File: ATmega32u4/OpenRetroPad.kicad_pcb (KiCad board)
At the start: 2 copper layers, 46 x 74 mm, 56 parts, among them J1 USB_C_Receptacle_USB2.0, J2 NRF24, J3 DB25_Female_MountingHoles, J4 USB_C_Receptacle_USB2.0, SW1 SW_Push, SW2 SW_Push, U1 ATmega32U4, U2 AMS1117-3.3, U3 CH330N, Y1 16MHz

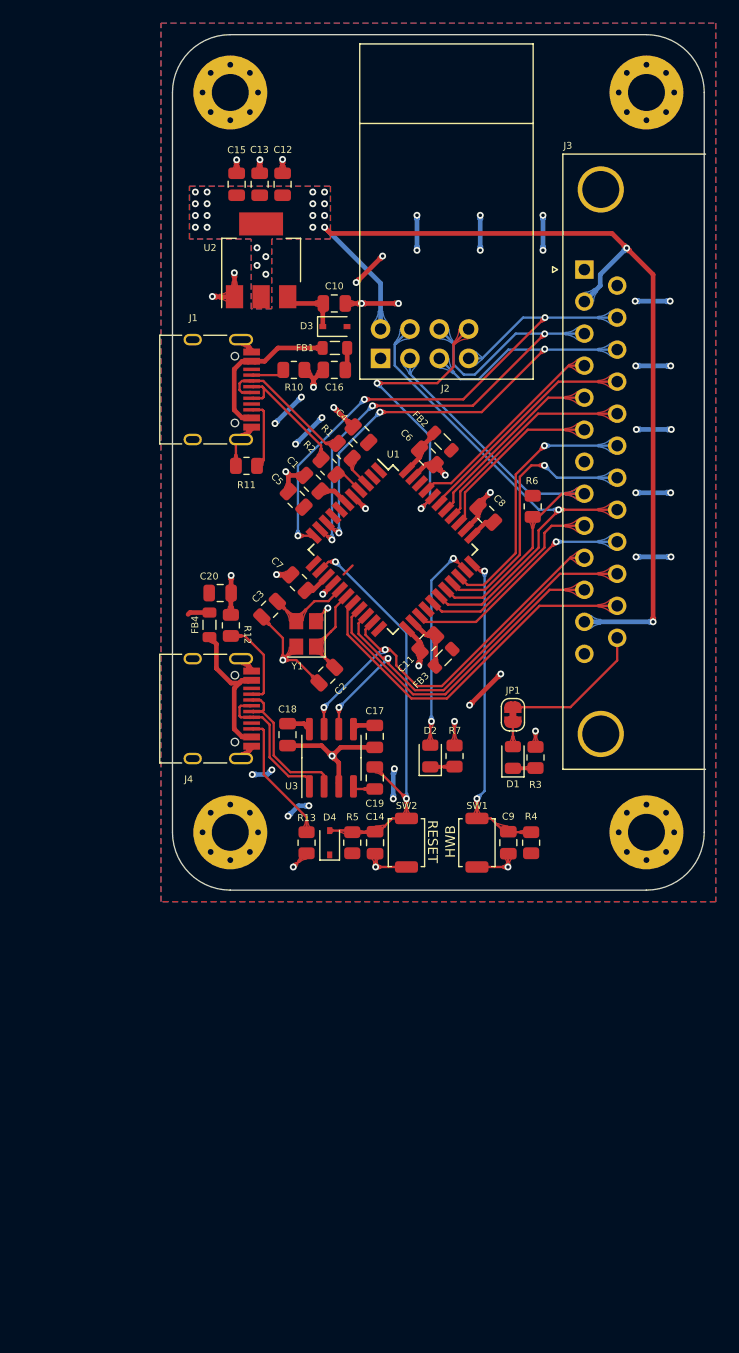
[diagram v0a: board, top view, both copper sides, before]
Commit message: Update V2
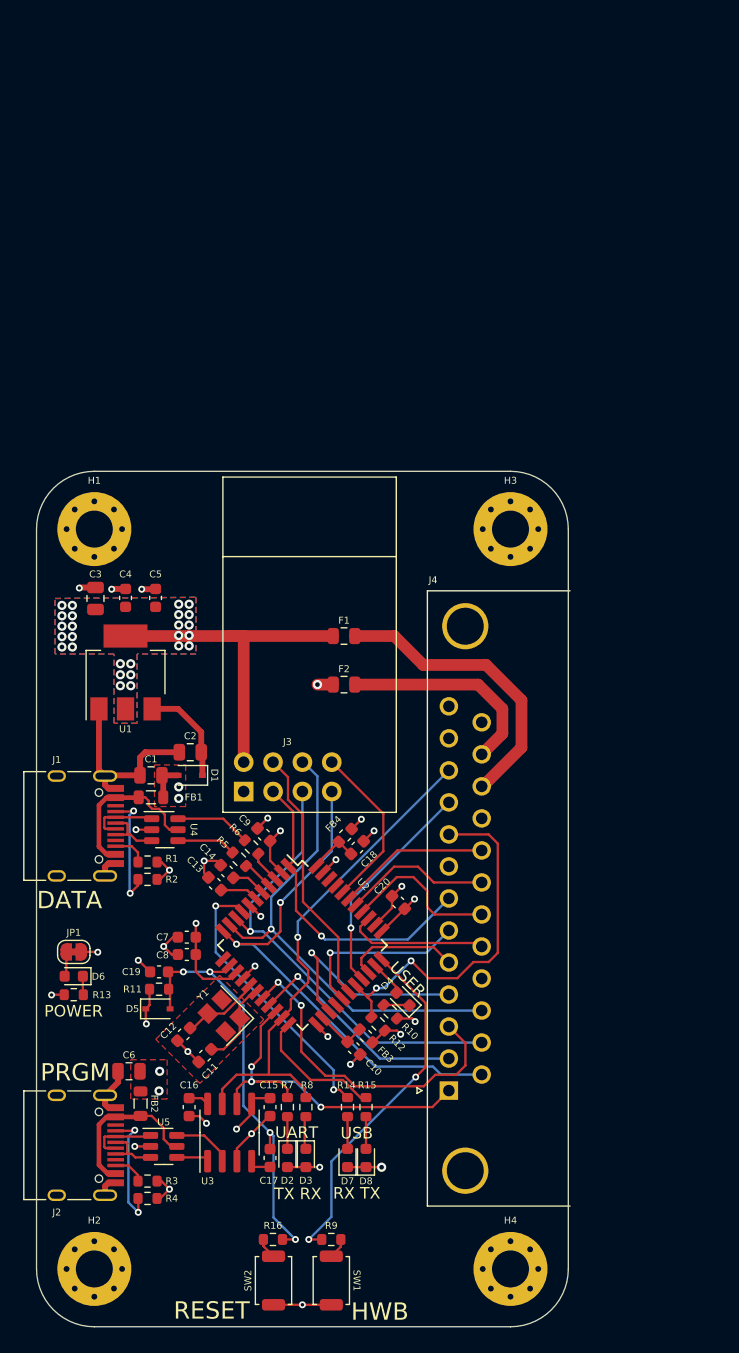
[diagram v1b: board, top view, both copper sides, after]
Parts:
- added D5: 1N5817, Diode_SMD:D_SOD-323, F.Cu at (105.5, 141.5)
- added D6: Power, LED_SMD:LED_0603_1608Metric, F.Cu at (98.2, 138.7)
- added D7: RX, LED_SMD:LED_0603_1608Metric, F.Cu at (121.9, 154.4)
- added D8: TX, LED_SMD:LED_0603_1608Metric, F.Cu at (123.5, 154.4)
- added F1: 500mA, Fuse:Fuse_0805_2012Metric, F.Cu at (121.6, 109.2)
- added F2: 500mA, Fuse:Fuse_0805_2012Metric, F.Cu at (121.6, 113.5)
- added R14: 1k, Resistor_SMD:R_0603_1608Metric, F.Cu at (121.9, 150.0)
- added R15: 1k, Resistor_SMD:R_0603_1608Metric, F.Cu at (123.5, 150.0)
- added R16: 330, Resistor_SMD:R_0603_1608Metric, F.Cu at (115.5, 161.4)
- added R8: 1k, Resistor_SMD:R_0603_1608Metric, F.Cu at (118.3, 150.0)
- added R9: 330, Resistor_SMD:R_0603_1608Metric, F.Cu at (120.5, 161.4)
- added U4: USBLC6-2SC6, Package_TO_SOT_SMD:SOT-23-6, F.Cu at (106.1, 126.0)
- added U5: USBLC6-2SC6, Package_TO_SOT_SMD:SOT-23-6, F.Cu at (106.0, 153.4)
- C1: value 1u -> 10u
- C10, C16, C20: value 10u -> 100n; footprint Capacitor_SMD:C_0805_2012Metric -> Capacitor_SMD:C_0603_1608Metric
- C11: value 100n -> 20pF; footprint Capacitor_SMD:C_0805_2012Metric -> Capacitor_SMD:C_0603_1608Metric
- C12: value 10u -> 20pF; footprint Capacitor_SMD:C_0805_2012Metric -> Capacitor_SMD:C_0603_1608Metric
- C13, C15, C17, C18, C19, C4, C8, C9: footprint Capacitor_SMD:C_0805_2012Metric -> Capacitor_SMD:C_0603_1608Metric
- C14, C7: value 100n -> 1u; footprint Capacitor_SMD:C_0805_2012Metric -> Capacitor_SMD:C_0603_1608Metric
- C2, C3: value 20pF -> 10u
- C5: value 1u -> 100n; footprint Capacitor_SMD:C_0805_2012Metric -> Capacitor_SMD:C_0603_1608Metric
- C6: value 100n -> 10u
- D1: value Power LED -> 1N5817; footprint LED_SMD:LED_0805_2012Metric -> Diode_SMD:D_SOD-323
- D2: value LED1 -> TX; footprint LED_SMD:LED_0805_2012Metric -> LED_SMD:LED_0603_1608Metric
- D3: value 1N5817 -> RX; footprint Diode_SMD:D_SOD-323 -> LED_SMD:LED_0603_1608Metric
- D4: value 1N5817 -> User; footprint Diode_SMD:D_SOD-323 -> LED_SMD:LED_0603_1608Metric
- FB3, FB4: footprint Inductor_SMD:L_0805_2012Metric -> Inductor_SMD:L_0603_1608Metric
- H1, H2, H3, H4: value 3.2mm_M3 -> 3.2mm M3
- J2: value NRF24 -> USB_C_Receptacle_USB2.0; footprint OpenRetroPad:NRF24L01 -> Connector_USB:USB_C_Receptacle_HRO_TYPE-C-31-M-12
- J3: value DB25_Female_MountingHoles -> NRF24; footprint Connector_Dsub:DSUB-25_Female_Horizontal_P2.77x2.84mm_EdgePinOffset7.70mm_Housed_MountingHolesOffset9.12mm -> OpenRetroPad:NRF24L01
- J4: value USB_C_Receptacle_USB2.0 -> DB25_Male_MountingHoles; footprint Connector_USB:USB_C_Receptacle_HRO_TYPE-C-31-M-12 -> Connector_Dsub:DSUB-25_Male_Horizontal_P2.77x2.84mm_EdgePinOffset7.70mm_Housed_MountingHolesOffset9.12mm
- R1, R2: value 22r -> 5.1k; footprint Resistor_SMD:R_0805_2012Metric -> Resistor_SMD:R_0603_1608Metric
- R10, R12, R13: value 5.1k -> 1k; footprint Resistor_SMD:R_0805_2012Metric -> Resistor_SMD:R_0603_1608Metric
- R11: value 5.1k -> 10k; footprint Resistor_SMD:R_0805_2012Metric -> Resistor_SMD:R_0603_1608Metric
- R3: value 1k -> 5.1k; footprint Resistor_SMD:R_0805_2012Metric -> Resistor_SMD:R_0603_1608Metric
- R4: value 10k -> 5.1k; footprint Resistor_SMD:R_0805_2012Metric -> Resistor_SMD:R_0603_1608Metric
- R5: value 10k -> 22r; footprint Resistor_SMD:R_0805_2012Metric -> Resistor_SMD:R_0603_1608Metric
- R6: value 1k -> 22r; footprint Resistor_SMD:R_0805_2012Metric -> Resistor_SMD:R_0603_1608Metric
- R7: footprint Resistor_SMD:R_0805_2012Metric -> Resistor_SMD:R_0603_1608Metric
- SW1: value SW_Push -> HWB
- SW2: value SW_Push -> RESET
- U1: value ATmega32U4 -> AMS1117-3.3; footprint Package_QFP:TQFP-44_10x10mm_P0.8mm -> Package_TO_SOT_SMD:SOT-223-3_TabPin2
- U2: value AMS1117-3.3 -> ATmega32U4-M; footprint Package_TO_SOT_SMD:SOT-223-3_TabPin2 -> Package_QFP:TQFP-44_10x10mm_P0.8mm
- moved H2 112.4 mm to (100.0, 164.0)
- moved C15 79.9 mm to (115.2, 150.0), turned to 90 degrees
- moved C12 74.0 mm to (107.7, 143.7), turned to -135 degrees
- moved J2 73.2 mm to (97.8, 153.3), turned to -90 degrees
- moved D3 72.0 mm to (118.3, 154.4), turned to -90 degrees
- moved C16 65.0 mm to (108.2, 150.0), turned to 90 degrees
- moved C10 64.4 mm to (122.5, 144.9), turned to 135 degrees
- moved FB2 63.0 mm to (104.0, 149.7), turned to 90 degrees
- moved C13 60.6 mm to (110.4, 130.7), turned to -45 degrees
- moved U2 59.4 mm to (118.0, 136.0), turned to -45 degrees
- moved C6 59.1 mm to (103.0, 146.9), turned to 0 degrees
- moved R10 56.1 mm to (125.6, 141.8), turned to 135 degrees
- moved J3 53.9 mm to (112.9, 122.7)
- moved R3 49.7 mm to (104.6, 156.4), turned to 0 degrees
- moved LOGO1 46.3 mm to (109.1, 164.1)
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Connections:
- C1 pad 2: Net-(C1-Pad2) -> +5V
- C10 pad 2: Net-(C10-Pad2) -> /Microcontroller/AVCC_P24
- C11 pad 1: GND -> /Microcontroller/XTAL1
- C11 pad 2: Net-(C11-Pad2) -> GND
- C12 pad 1: GND -> /Microcontroller/XTAL2
- C12 pad 2: +3V3 -> GND
- C13 pad 2: +3V3 -> /Microcontroller/UCAP
- C14 pad 1: RESET -> GND
- C14 pad 2: GND -> /Microcontroller/UGND
- C15 pad 2: +3V3 -> +5V
- C16 pad 2: +5V -> /UART/V3
- C17 pad 1: GND -> /UART/RTS
- C17 pad 2: +5V -> /DB25/RST
- C18 pad 2: Net-(C18-Pad2) -> /Microcontroller/AVCC_P44
- C19 pad 1: Net-(C19-Pad1) -> /DB25/RST
- C19 pad 2: RESET -> GND
- C2 pad 1: XTAL1 -> GND
- C2 pad 2: GND -> /Power/VREGIN
- C3 pad 1: XTAL2 -> GND
- C3 pad 2: GND -> +3V3
- C4 pad 2: +5V -> +3V3
- C5 pad 2: +5V -> +3V3
- C6 pad 2: Net-(C6-Pad2) -> +5V
- C9 pad 1: PE2 -> GND
- C9 pad 2: GND -> +5V
- D1 pad 1: Net-(D1-Pad1) -> /Power/VREGIN
- D1 pad 2: Net-(D1-Pad2) -> +5V
- D2 pad 2: PC7 -> +5V
- D3 pad 1: Net-(C10-Pad2) -> Net-(D3-Pad1)
- D4 pad 1: +5V -> Net-(D4-Pad1)
- D4 pad 2: RESET -> /IO/LED_USER
- FB1 pad 1: +5V -> /USB Data/VBUS
- FB1 pad 2: Net-(FB1-Pad2) -> +5V
- FB2 pad 1: +5V -> /USB Program/VBUS
- FB2 pad 2: Net-(C6-Pad2) -> +5V
- FB3 pad 1: +5V -> /Microcontroller/AVCC_P24
- FB3 pad 2: Net-(C11-Pad2) -> +5V
- FB4 pad 1: +5V -> /Microcontroller/AVCC_P44
- FB4 pad 2: Net-(FB4-Pad2) -> +5V
- H1 pad 1: (no net) -> unconnected-(H1-Pad1)
- H2 pad 1: (no net) -> unconnected-(H2-Pad1)
- H3 pad 1: (no net) -> unconnected-(H3-Pad1)
- H4 pad 1: (no net) -> unconnected-(H4-Pad1)
- J1 pad A4: Net-(FB1-Pad2) -> /USB Data/VBUS
- J1 pad A5: Net-(J1-PadA5) -> /USB Data/CC1
- J1 pad A6: MCU_D+ -> /USB Data/D+
- J1 pad A7: MCU_D- -> /USB Data/D-
- J1 pad A8: Net-(J1-PadA8) -> unconnected-(J1-PadA8)
- J1 pad A9: Net-(FB1-Pad2) -> /USB Data/VBUS
- J1 pad B4: Net-(FB1-Pad2) -> /USB Data/VBUS
- J1 pad B5: Net-(J1-PadB5) -> /USB Data/CC2
- J1 pad B6: MCU_D+ -> /USB Data/D+
- J1 pad B7: MCU_D- -> /USB Data/D-
- J1 pad B8: Net-(J1-PadB8) -> unconnected-(J1-PadB8)
- J1 pad B9: Net-(FB1-Pad2) -> /USB Data/VBUS
- J3 pad 3: PB2 -> /DB25/CE
- J3 pad 4: PF0 -> /DB25/CSN
- J3 pad 5: PF5 -> /DB25/SCK
- J3 pad 6: PF7 -> /DB25/MOSI
- J3 pad 7: Net-(J3-Pad7) -> /DB25/MISO
- J3 pad 8: PB5 -> /DB25/IRQ
- JP1 pad 2: Net-(D1-Pad2) -> Net-(D6-Pad2)
- R1 pad 1: Net-(R1-Pad1) -> /USB Data/CC2
- R1 pad 2: MCU_D- -> GND
- R10 pad 2: Net-(J1-PadA5) -> Net-(D4-Pad1)
- R11 pad 1: Net-(J1-PadB5) -> +5V
- R11 pad 2: GND -> /DB25/RST
- R12 pad 1: GND -> /DB25/PB5
- R12 pad 2: Net-(J4-PadA5) -> +5V
- R13 pad 1: Net-(J4-PadB5) -> Net-(D6-Pad1)
- R2 pad 1: Net-(R2-Pad1) -> GND
- R2 pad 2: MCU_D+ -> /USB Data/CC1
- R3 pad 1: Net-(D1-Pad1) -> /USB Program/CC2
- R4 pad 1: +5V -> GND
- R4 pad 2: PE2 -> /USB Program/CC1
- R5 pad 1: +5V -> /Microcontroller/D+
- R5 pad 2: RESET -> /Microcontroller/USB_DATA.DP
- R6 pad 1: PB5 -> /Microcontroller/D-
- R6 pad 2: +5V -> /Microcontroller/USB_DATA.DM
- R7 pad 1: GND -> Net-(D2-Pad1)
- R7 pad 2: Net-(D2-Pad1) -> /DB25/TX
- SW1 pad 1: PE2 -> Net-(R9-Pad2)
- SW2 pad 1: RESET -> Net-(R16-Pad2)
- U1 pad 1: Net-(U1-Pad1) -> GND
- U1 pad 2: +5V -> +3V3
- U1 pad 3: Net-(R1-Pad1) -> /Power/VREGIN
- U2 pad 1: GND -> /DB25/CE
- U2 pad 2: +3V3 -> +5V
- U2 pad 3: Net-(C10-Pad2) -> /Microcontroller/D-
- U3 pad 1: /UART_D+ -> /UART/USB_PRGM.DP
- U3 pad 2: /UART_D- -> /UART/USB_PRGM.DM
- U3 pad 4: Net-(C19-Pad1) -> /UART/RTS
- U3 pad 6: PD2 -> /DB25/TX
- U3 pad 7: PD3 -> /DB25/RX
- U3 pad 8: Net-(C18-Pad2) -> /UART/V3
- Y1 pad 1: XTAL1 -> /Microcontroller/XTAL1
- Y1 pad 3: XTAL2 -> /Microcontroller/XTAL2
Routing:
- net +3V3: track 83.6 -> 30.2 mm, vias 22 -> 26
- net PB2: track 48.7 -> 0.00 mm, vias 3 -> 0
- net PB3: track 48.4 -> 0.00 mm, vias 3 -> 0
- net PB1: track 47.0 -> 0.00 mm, vias 3 -> 0
- net /DB25/MISO: track 0.00 -> 45.7 mm, vias 0 -> 2
- net /DB25/RX: track 0.00 -> 43.7 mm, vias 0 -> 1
- net PB4: track 43.0 -> 0.00 mm, vias 1 -> 0
- net /DB25/MOSI: track 0.00 -> 42.1 mm, vias 0 -> 1
- net /DB25/SCK: track 0.00 -> 39.7 mm, vias 0 -> 1
- net PD2: track 38.5 -> 0.00 mm, vias 2 -> 0
- net PB5: track 38.3 -> 0.00 mm
- net RESET: track 37.7 -> 0.00 mm, vias 2 -> 0
- net /DB25/RST: track 0.00 -> 37.6 mm, vias 0 -> 4
- net PD3: track 36.4 -> 0.00 mm, vias 2 -> 0
- net /DB25/TX: track 0.00 -> 32.4 mm, vias 0 -> 3
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- added copper zone on In2.Cu, net +5V
- added copper zone on F.Cu, net GND
- added copper zone on In1.Cu, net GND
- removed copper zone on B.Cu, net GND
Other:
- copper layers 2 -> 4
- net class Default removed
- board text added: "DATA"
- board text added: "OpenRetroPad ATmega32u4 v2 DEC-2022 OpenRetroPad.com JLCJLCJLCJLC"
- board text added: "POWER"
- board text added: "PRGM"
- board text added: "RX TX"
- board text added: "TX RX"
- board text added: "UART"
- board text added: "USB"
- board text added: "USER"
- board text removed: "1 14 2 15 3 16 4 17 5 18 6 19 7 20 8 21 9 22 10 23 11 24 12 25 13"
- board text removed: "3V3 GND"
- board text removed: "ATmega32u4"
- board text removed: "DB25"
- board text removed: "GND 5V 3V3 PB3 PB2 PB1 PF0 PF4 PF5 PF6 PF7 PC6 - PB6 PB5 PB4 PD7 PD4 PD3 PD2 PD1 PD0 3V3 5V GND"
- board text removed: "OpenRetroPad ATmega32u4 v1 MAY-2021 OpenRetroPad.com JLCJLCJLCJLC"
- board text removed: "PB2 PB1"
- board text removed: "PB4 PB5"
- board text removed: "PF1 PB3"
